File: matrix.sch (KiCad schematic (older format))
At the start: 8 parts

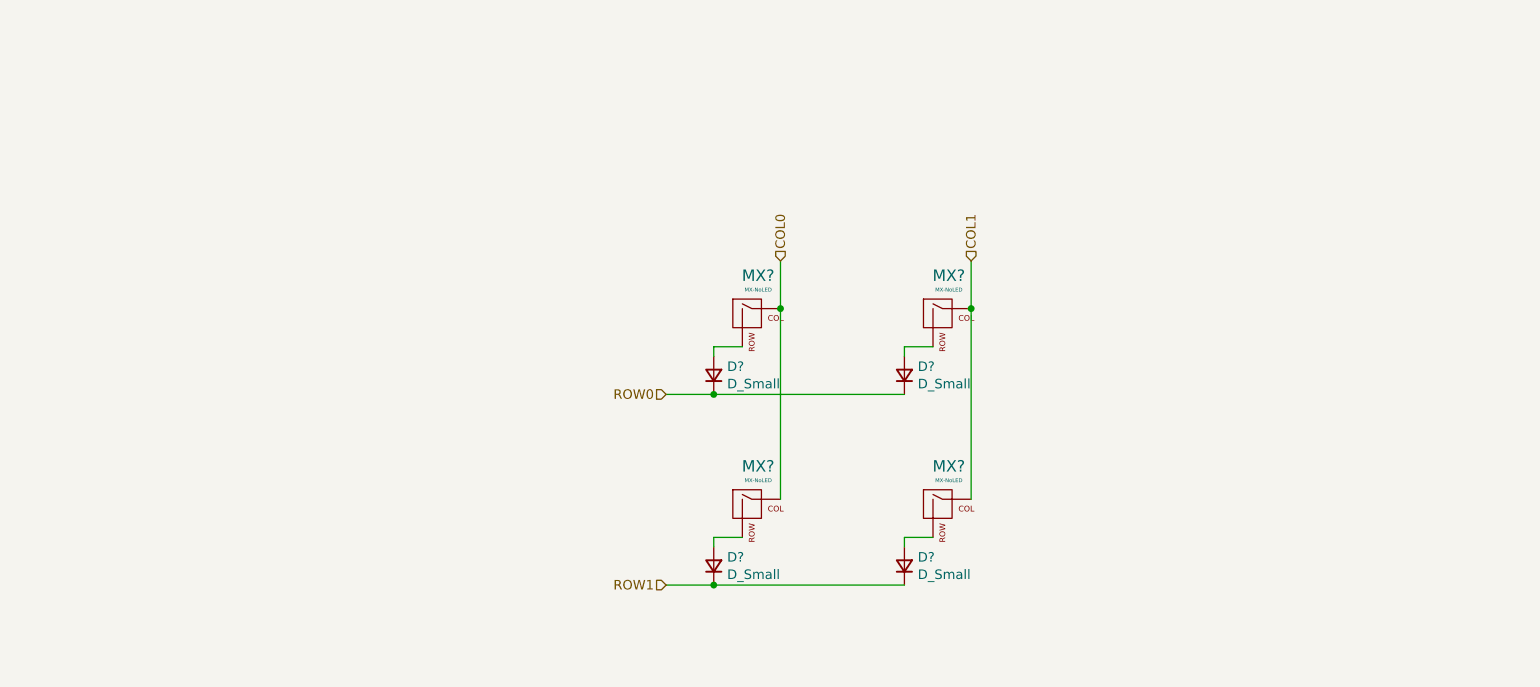
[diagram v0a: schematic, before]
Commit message: update matrix
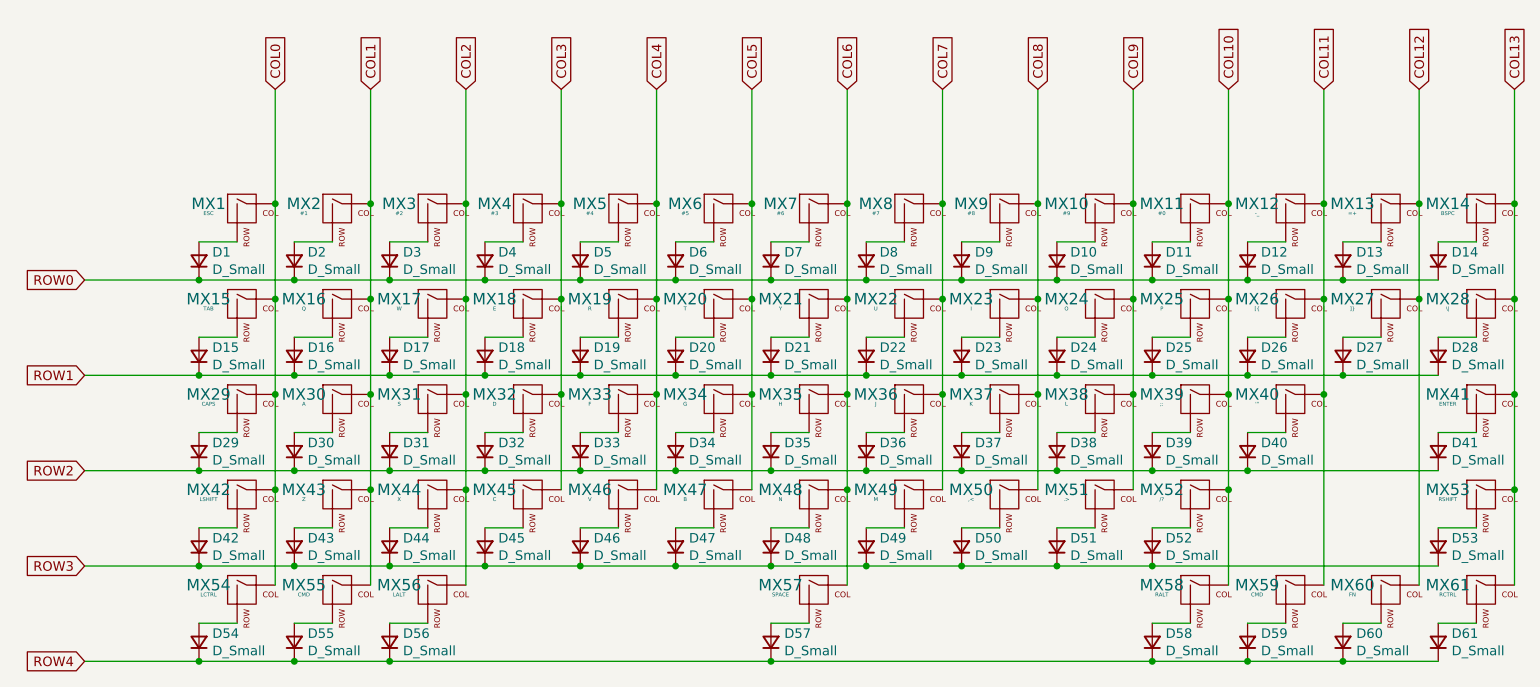
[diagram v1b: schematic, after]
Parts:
- removed D? (x4): D_Small, Diode_SMD:D_SOD-123, symbol Device:D_Small
- removed MX? (x4): MX-NoLED, MX_Alps_Hybrid:MX-1U, symbol MX_Alps_Hybrid:MX-NoLED
- added D1, D10, D11, D12, D13, D14, D15, D16, D17, D18, D19, D2, D20, D21, D22, D23, D24, D25, D26, D27, D28, D29, D3, D30, D31, D32, D33, D34, D35, D36, D37, D38, D39, D4, D40, D41, D42, D43, D44, D45, D46, D47, D48, D49, D5, D50, D51, D52, D53, D54, D55, D56, D57, D58, D59, D6, D60, D61, D7, D8, D9: D_Small, Diode_SMD:D_SOD-123, symbol Device:D_Small
- added MX1: ESC, MX_Alps_Hybrid:MX-1U, symbol MX_Alps_Hybrid:MX-NoLED
- added MX10: #9, MX_Alps_Hybrid:MX-1U, symbol MX_Alps_Hybrid:MX-NoLED
- added MX11: #0, MX_Alps_Hybrid:MX-1U, symbol MX_Alps_Hybrid:MX-NoLED
- added MX12: -_, MX_Alps_Hybrid:MX-1U, symbol MX_Alps_Hybrid:MX-NoLED
- added MX13: =+, MX_Alps_Hybrid:MX-1U, symbol MX_Alps_Hybrid:MX-NoLED
- added MX14: BSPC, MX_Alps_Hybrid:MX-1U, symbol MX_Alps_Hybrid:MX-NoLED
- added MX15: TAB, MX_Alps_Hybrid:MX-1U, symbol MX_Alps_Hybrid:MX-NoLED
- added MX16: Q, MX_Alps_Hybrid:MX-1U, symbol MX_Alps_Hybrid:MX-NoLED
- added MX17: W, MX_Alps_Hybrid:MX-1U, symbol MX_Alps_Hybrid:MX-NoLED
- added MX18: E, MX_Alps_Hybrid:MX-1U, symbol MX_Alps_Hybrid:MX-NoLED
- added MX19: R, MX_Alps_Hybrid:MX-1U, symbol MX_Alps_Hybrid:MX-NoLED
- added MX2: #1, MX_Alps_Hybrid:MX-1U, symbol MX_Alps_Hybrid:MX-NoLED
- added MX20: T, MX_Alps_Hybrid:MX-1U, symbol MX_Alps_Hybrid:MX-NoLED
- added MX21: Y, MX_Alps_Hybrid:MX-1U, symbol MX_Alps_Hybrid:MX-NoLED
- added MX22: U, MX_Alps_Hybrid:MX-1U, symbol MX_Alps_Hybrid:MX-NoLED
- added MX23: I, MX_Alps_Hybrid:MX-1U, symbol MX_Alps_Hybrid:MX-NoLED
- added MX24: O, MX_Alps_Hybrid:MX-1U, symbol MX_Alps_Hybrid:MX-NoLED
- added MX25: P, MX_Alps_Hybrid:MX-1U, symbol MX_Alps_Hybrid:MX-NoLED
- added MX26: [{, MX_Alps_Hybrid:MX-1U, symbol MX_Alps_Hybrid:MX-NoLED
- added MX27: ]}, MX_Alps_Hybrid:MX-1U, symbol MX_Alps_Hybrid:MX-NoLED
- added MX28: \\|, MX_Alps_Hybrid:MX-1U, symbol MX_Alps_Hybrid:MX-NoLED
- added MX29: CAPS, MX_Alps_Hybrid:MX-1U, symbol MX_Alps_Hybrid:MX-NoLED
- added MX3: #2, MX_Alps_Hybrid:MX-1U, symbol MX_Alps_Hybrid:MX-NoLED
- added MX30: A, MX_Alps_Hybrid:MX-1U, symbol MX_Alps_Hybrid:MX-NoLED
- added MX31: S, MX_Alps_Hybrid:MX-1U, symbol MX_Alps_Hybrid:MX-NoLED
- added MX32: D, MX_Alps_Hybrid:MX-1U, symbol MX_Alps_Hybrid:MX-NoLED
- added MX33: F, MX_Alps_Hybrid:MX-1U, symbol MX_Alps_Hybrid:MX-NoLED
- added MX34: G, MX_Alps_Hybrid:MX-1U, symbol MX_Alps_Hybrid:MX-NoLED
- added MX35: H, MX_Alps_Hybrid:MX-1U, symbol MX_Alps_Hybrid:MX-NoLED
- added MX36: J, MX_Alps_Hybrid:MX-1U, symbol MX_Alps_Hybrid:MX-NoLED
- added MX37: K, MX_Alps_Hybrid:MX-1U, symbol MX_Alps_Hybrid:MX-NoLED
- added MX38: L, MX_Alps_Hybrid:MX-1U, symbol MX_Alps_Hybrid:MX-NoLED
- added MX39: ;:, MX_Alps_Hybrid:MX-1U, symbol MX_Alps_Hybrid:MX-NoLED
- added MX4: #3, MX_Alps_Hybrid:MX-1U, symbol MX_Alps_Hybrid:MX-NoLED
- added MX40: '\", MX_Alps_Hybrid:MX-1U, symbol MX_Alps_Hybrid:MX-NoLED
- added MX41: ENTER, MX_Alps_Hybrid:MX-1U, symbol MX_Alps_Hybrid:MX-NoLED
- added MX42: LSHIFT, MX_Alps_Hybrid:MX-1U, symbol MX_Alps_Hybrid:MX-NoLED
- added MX43: Z, MX_Alps_Hybrid:MX-1U, symbol MX_Alps_Hybrid:MX-NoLED
- added MX44: X, MX_Alps_Hybrid:MX-1U, symbol MX_Alps_Hybrid:MX-NoLED
- added MX45: C, MX_Alps_Hybrid:MX-1U, symbol MX_Alps_Hybrid:MX-NoLED
- added MX46: V, MX_Alps_Hybrid:MX-1U, symbol MX_Alps_Hybrid:MX-NoLED
- added MX47: B, MX_Alps_Hybrid:MX-1U, symbol MX_Alps_Hybrid:MX-NoLED
- added MX48: N, MX_Alps_Hybrid:MX-1U, symbol MX_Alps_Hybrid:MX-NoLED
- added MX49: M, MX_Alps_Hybrid:MX-1U, symbol MX_Alps_Hybrid:MX-NoLED
- added MX5: #4, MX_Alps_Hybrid:MX-1U, symbol MX_Alps_Hybrid:MX-NoLED
- added MX50: ,<, MX_Alps_Hybrid:MX-1U, symbol MX_Alps_Hybrid:MX-NoLED
- added MX51: .>, MX_Alps_Hybrid:MX-1U, symbol MX_Alps_Hybrid:MX-NoLED
- added MX52: /?, MX_Alps_Hybrid:MX-1U, symbol MX_Alps_Hybrid:MX-NoLED
- added MX53: RSHIFT, MX_Alps_Hybrid:MX-1U, symbol MX_Alps_Hybrid:MX-NoLED
- added MX54: LCTRL, MX_Alps_Hybrid:MX-1U, symbol MX_Alps_Hybrid:MX-NoLED
- added MX55, MX59: CMD, MX_Alps_Hybrid:MX-1U, symbol MX_Alps_Hybrid:MX-NoLED
- added MX56: LALT, MX_Alps_Hybrid:MX-1U, symbol MX_Alps_Hybrid:MX-NoLED
- added MX57: SPACE, MX_Alps_Hybrid:MX-1U, symbol MX_Alps_Hybrid:MX-NoLED
- added MX58: RALT, MX_Alps_Hybrid:MX-1U, symbol MX_Alps_Hybrid:MX-NoLED
- added MX6: #5, MX_Alps_Hybrid:MX-1U, symbol MX_Alps_Hybrid:MX-NoLED
- added MX60: FN, MX_Alps_Hybrid:MX-1U, symbol MX_Alps_Hybrid:MX-NoLED
- added MX61: RCTRL, MX_Alps_Hybrid:MX-1U, symbol MX_Alps_Hybrid:MX-NoLED
- added MX7: #6, MX_Alps_Hybrid:MX-1U, symbol MX_Alps_Hybrid:MX-NoLED
- added MX8: #7, MX_Alps_Hybrid:MX-1U, symbol MX_Alps_Hybrid:MX-NoLED
- added MX9: #8, MX_Alps_Hybrid:MX-1U, symbol MX_Alps_Hybrid:MX-NoLED
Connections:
- net COL0: now also MX1.1 (COL), MX15.1 (COL), MX29.1 (COL), MX42.1 (COL), MX54.1 (COL)
- net COL1: now also MX16.1 (COL), MX2.1 (COL), MX30.1 (COL), MX43.1 (COL), MX55.1 (COL)
- net ROW0: now also D1.1 (K), D10.1 (K), D11.1 (K), D12.1 (K), D13.1 (K), D14.1 (K), D2.1 (K), D3.1 (K), D4.1 (K), D5.1 (K), D6.1 (K), D7.1 (K), D8.1 (K), D9.1 (K)
- net ROW1: now also D15.1 (K), D16.1 (K), D17.1 (K), D18.1 (K), D19.1 (K), D20.1 (K), D21.1 (K), D22.1 (K), D23.1 (K), D24.1 (K), D25.1 (K), D26.1 (K), D27.1 (K), D28.1 (K)
- new net: D1.2 (A), MX1.2 (ROW)
- new net: D2.2 (A), MX2.2 (ROW)
- new net: D3.2 (A), MX3.2 (ROW)
- new net: D15.2 (A), MX15.2 (ROW)
- new net: D16.2 (A), MX16.2 (ROW)
- new net: D17.2 (A), MX17.2 (ROW)
- new net: D29.2 (A), MX29.2 (ROW)
- new net: D30.2 (A), MX30.2 (ROW)
- new net: D31.2 (A), MX31.2 (ROW)
- new net: D4.2 (A), MX4.2 (ROW)
- new net: D5.2 (A), MX5.2 (ROW)
- new net: D6.2 (A), MX6.2 (ROW)
- new net: D18.2 (A), MX18.2 (ROW)
- new net: D19.2 (A), MX19.2 (ROW)
- new net: D20.2 (A), MX20.2 (ROW)
- new net: D32.2 (A), MX32.2 (ROW)
- new net: D33.2 (A), MX33.2 (ROW)
- new net: D34.2 (A), MX34.2 (ROW)
- new net: D7.2 (A), MX7.2 (ROW)
- new net: D8.2 (A), MX8.2 (ROW)
- new net: D9.2 (A), MX9.2 (ROW)
- new net: D21.2 (A), MX21.2 (ROW)
- new net: D22.2 (A), MX22.2 (ROW)
- new net: D23.2 (A), MX23.2 (ROW)
- new net: D35.2 (A), MX35.2 (ROW)
- new net: D36.2 (A), MX36.2 (ROW)
- new net: D37.2 (A), MX37.2 (ROW)
- new net: D10.2 (A), MX10.2 (ROW)
- new net: D11.2 (A), MX11.2 (ROW)
- new net: D12.2 (A), MX12.2 (ROW)
- new net: D24.2 (A), MX24.2 (ROW)
- new net: D25.2 (A), MX25.2 (ROW)
- new net: D26.2 (A), MX26.2 (ROW)
- new net: D38.2 (A), MX38.2 (ROW)
- new net: D39.2 (A), MX39.2 (ROW)
- new net: D40.2 (A), MX40.2 (ROW)
- new net: D13.2 (A), MX13.2 (ROW)
- new net: D14.2 (A), MX14.2 (ROW)
- new net: D27.2 (A), MX27.2 (ROW)
- new net: D28.2 (A), MX28.2 (ROW)
- new net: D41.2 (A), MX41.2 (ROW)
- new net: D42.2 (A), MX42.2 (ROW)
- new net: D43.2 (A), MX43.2 (ROW)
- new net: D44.2 (A), MX44.2 (ROW)
- new net: D54.2 (A), MX54.2 (ROW)
- new net: D55.2 (A), MX55.2 (ROW)
- new net: D56.2 (A), MX56.2 (ROW)
- new net: D45.2 (A), MX45.2 (ROW)
- new net: D46.2 (A), MX46.2 (ROW)
- new net: D47.2 (A), MX47.2 (ROW)
- new net: D48.2 (A), MX48.2 (ROW)
- new net: D49.2 (A), MX49.2 (ROW)
- new net: D50.2 (A), MX50.2 (ROW)
- new net: D57.2 (A), MX57.2 (ROW)
- new net: D51.2 (A), MX51.2 (ROW)
- new net: D52.2 (A), MX52.2 (ROW)
- new net: D58.2 (A), MX58.2 (ROW)
- new net: D59.2 (A), MX59.2 (ROW)
- new net: D53.2 (A), MX53.2 (ROW)
- new net: D60.2 (A), MX60.2 (ROW)
- new net: D61.2 (A), MX61.2 (ROW)
- new net COL10: MX11.1 (COL), MX25.1 (COL), MX39.1 (COL), MX52.1 (COL), MX58.1 (COL)
- new net COL11: MX12.1 (COL), MX26.1 (COL), MX40.1 (COL), MX59.1 (COL)
- new net COL12: MX13.1 (COL), MX27.1 (COL), MX60.1 (COL)
- new net COL13: MX14.1 (COL), MX28.1 (COL), MX41.1 (COL), MX53.1 (COL), MX61.1 (COL)
- new net COL2: MX17.1 (COL), MX3.1 (COL), MX31.1 (COL), MX44.1 (COL), MX56.1 (COL)
- new net COL3: MX18.1 (COL), MX32.1 (COL), MX4.1 (COL), MX45.1 (COL)
- new net COL4: MX19.1 (COL), MX33.1 (COL), MX46.1 (COL), MX5.1 (COL)
- new net COL5: MX20.1 (COL), MX34.1 (COL), MX47.1 (COL), MX6.1 (COL)
- new net COL6: MX21.1 (COL), MX35.1 (COL), MX48.1 (COL), MX57.1 (COL), MX7.1 (COL)
- new net COL7: MX22.1 (COL), MX36.1 (COL), MX49.1 (COL), MX8.1 (COL)
- new net COL8: MX23.1 (COL), MX37.1 (COL), MX50.1 (COL), MX9.1 (COL)
- new net COL9: MX10.1 (COL), MX24.1 (COL), MX38.1 (COL), MX51.1 (COL)
- new net ROW2: D29.1 (K), D30.1 (K), D31.1 (K), D32.1 (K), D33.1 (K), D34.1 (K), D35.1 (K), D36.1 (K), D37.1 (K), D38.1 (K), D39.1 (K), D40.1 (K), D41.1 (K)
- new net ROW3: D42.1 (K), D43.1 (K), D44.1 (K), D45.1 (K), D46.1 (K), D47.1 (K), D48.1 (K), D49.1 (K), D50.1 (K), D51.1 (K), D52.1 (K), D53.1 (K)
- new net ROW4: D54.1 (K), D55.1 (K), D56.1 (K), D57.1 (K), D58.1 (K), D59.1 (K), D60.1 (K), D61.1 (K)
